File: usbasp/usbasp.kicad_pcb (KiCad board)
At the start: 2 copper layers, 80 x 50 mm, 25 parts, among them J1 USB_B, J2 AVR-ISP-10, J3 AVR-ISP-6, U1 ATmega8-16PU, Y1 12MHz

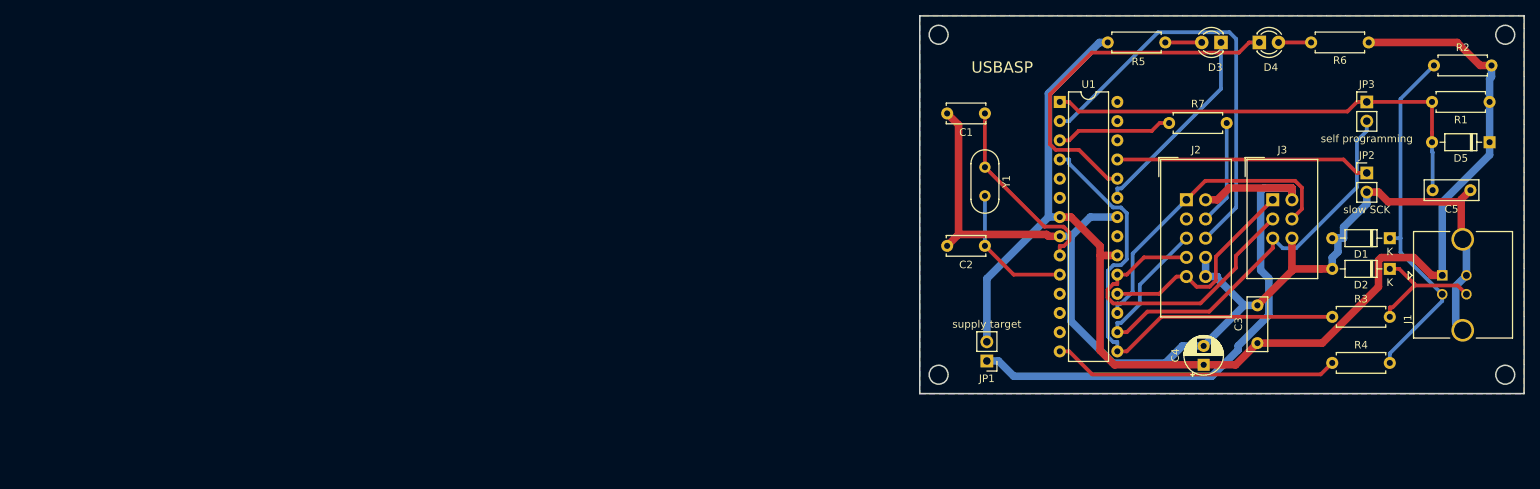
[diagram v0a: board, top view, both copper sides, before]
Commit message: update: new revision
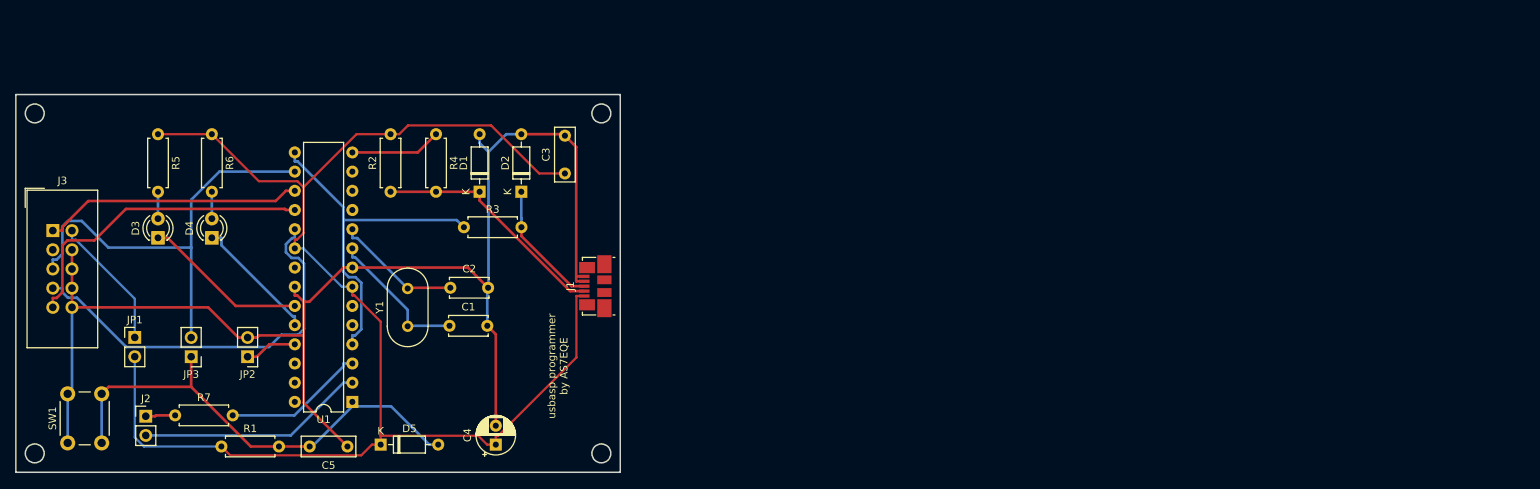
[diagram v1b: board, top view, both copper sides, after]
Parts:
- added SW1: RESET, Button_Switch_THT:SW_PUSH_6mm, F.Cu at (64.5, 109.9)
- J1: footprint Connector_USB:USB_B_TE_5787834_Vertical -> Connector_USB:USB_Micro-B_Molex_47346-0001
- J2: value AVR-ISP-10 -> TxD RxD; footprint Connector_IDC:IDC-Header_2x05_P2.54mm_Vertical -> Connector_PinHeader_2.54mm:PinHeader_1x02_P2.54mm_Vertical
- J3: value AVR-ISP-6 -> AVR-ISP-10; footprint Connector_IDC:IDC-Header_2x03_P2.54mm_Vertical -> Connector_IDC:IDC-Header_2x05_P2.54mm_Vertical
- Y1: footprint Crystal:Crystal_HC52-8mm_Vertical -> Crystal:Resonator-2Pin_W10.0mm_H5.0mm
- moved R1 174.0 mm to (84.9, 110.4), turned to 0 degrees
- moved J3 161.5 mm to (62.5, 81.8)
- moved JP3 159.2 mm to (80.9, 98.5), turned to 180 degrees
- moved R6 153.6 mm to (83.6, 69.0), turned to 270 degrees
- moved C5 152.5 mm to (101.5, 110.4)
- moved D5 152.1 mm to (105.9, 110.1), turned to 0 degrees
- moved JP2 150.1 mm to (88.3, 98.5), turned to 180 degrees
- moved R7 144.5 mm to (78.7, 106.3), turned to 0 degrees
- moved D3 143.1 mm to (76.5, 82.8), turned to 90 degrees
- moved D4 141.0 mm to (83.6, 82.8), turned to 90 degrees
- moved J2 140.7 mm to (74.9, 106.4)
- moved R2 139.1 mm to (107.3, 76.7), turned to 90 degrees
- moved R5 126.3 mm to (76.5, 69.0), turned to 270 degrees
- moved R4 122.4 mm to (113.3, 69.0), turned to 270 degrees
- moved D1 120.6 mm to (119.0, 76.7), turned to 90 degrees
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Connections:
- J2 pad 2: VCCINT -> Net-(J2-Pad2)
- J3 pad 1: Net-(J2-Pad9) -> Net-(J3-Pad1)
- J3 pad 3: Net-(J2-Pad7) -> Net-(J3-Pad3)
- J3 pad 4: Net-(J2-Pad1) -> GND
- J3 pad 5: Net-(J2-Pad5) -> Net-(J3-Pad5)
- JP3 pad 2: Net-(J2-Pad5) -> Net-(J3-Pad5)
- R7 pad 1: Net-(J2-Pad4) -> Net-(J2-Pad1)
- U1 pad 16: Net-(J2-Pad5) -> Net-(J3-Pad5)
- U1 pad 17: Net-(J2-Pad1) -> Net-(J3-Pad1)
- U1 pad 18: Net-(J2-Pad9) -> Net-(J3-Pad9)
- U1 pad 19: Net-(J2-Pad7) -> Net-(J3-Pad7)
- U1 pad 2: Net-(J2-Pad6) -> Net-(J2-Pad2)
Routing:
- net Net-(J2-Pad5): track 67.4 -> 0.00 mm
- net VCCINT: track 78.2 -> 17.9 mm
- net Net-(J3-Pad5): track 0.00 -> 58.7 mm
- net Net-(J2-Pad6): track 56.6 -> 0.00 mm
- net Net-(J3-Pad7): track 0.00 -> 53.2 mm
- net Net-(J3-Pad9): track 0.00 -> 41.8 mm
- net Net-(J2-Pad7): track 41.7 -> 0.00 mm
- net Net-(J2-Pad1): track 40.5 -> 3.93 mm
- net Net-(J3-Pad1): track 0.00 -> 34.5 mm
- net Net-(D4-Pad1): track 48.0 -> 17.0 mm
- net Net-(J2-Pad2): track 0.00 -> 30.2 mm
- net Net-(J2-Pad9): track 28.7 -> 0.00 mm
- net GND: track 154.4 -> 182.7 mm
- net Net-(JP2-Pad1): track 33.8 -> 6.93 mm
- net Net-(R4-Pad1): track 38.0 -> 12.1 mm
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- removed copper zone on B.Cu, net +5V
- removed copper zone on F.Cu, net GND
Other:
- outline, holes or cut-outs redrawn
- net class +5V added: clearance 0.2, trace_width 0.3, via_dia 0.8, via_drill 0.4
- net class GND added: clearance 0.2, trace_width 0.35, via_dia 0.8, via_drill 0.4
- net class power removed
- net class signals: trace_width 0.5 -> 0.35
- board text added: "usbasp programmer by AS7EQE"
- board text removed: "USBASP"
